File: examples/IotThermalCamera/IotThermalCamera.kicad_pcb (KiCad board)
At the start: 4 copper layers, 48 x 37 mm, 53 parts

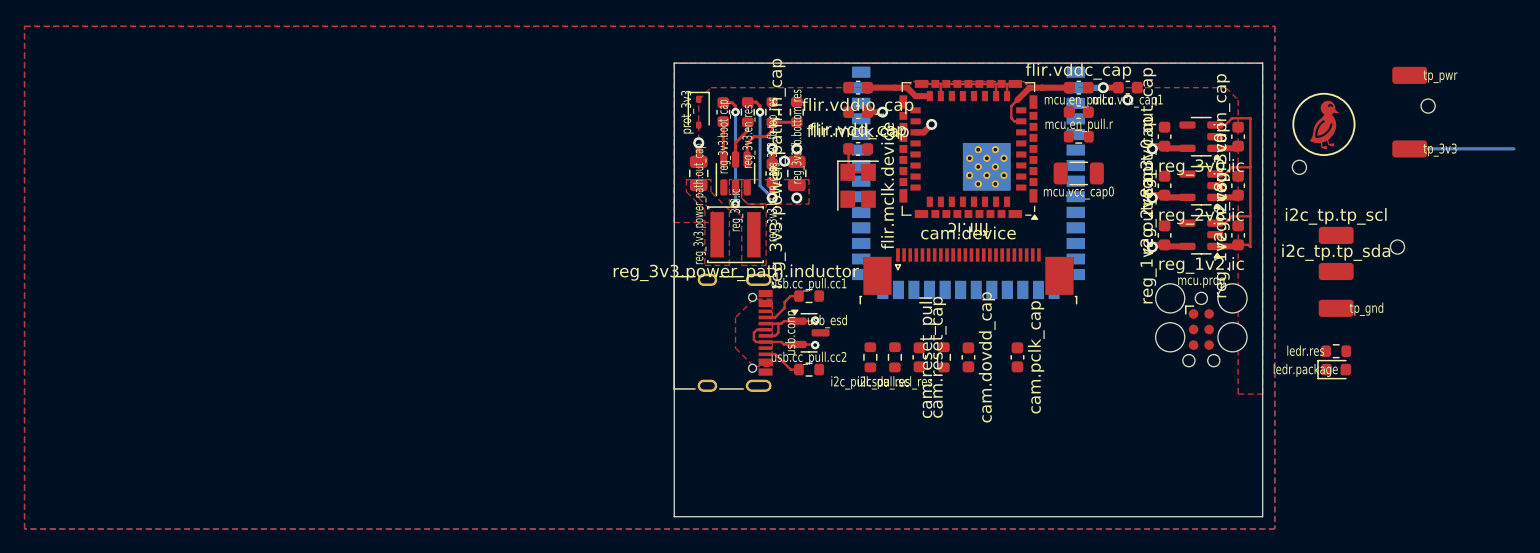
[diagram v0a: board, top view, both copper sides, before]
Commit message: Update IotThermalCamera.kicad_pcb
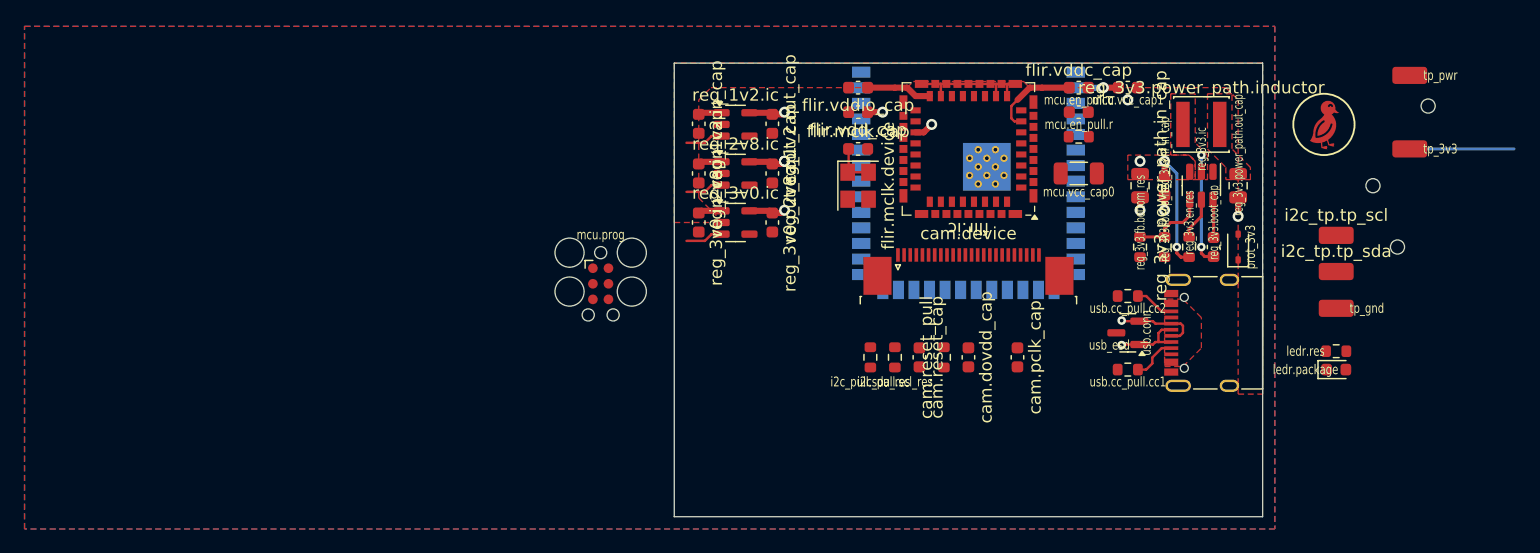
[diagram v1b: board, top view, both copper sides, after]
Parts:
- moved mcu.prog 49.1 mm to (120.0, 111.0)
- moved prot_3v3 45.4 mm to (172.0, 108.0), turned to 90 degrees
- moved reg_1v2.in_cap 44.9 mm to (128.0, 98.0), turned to -90 degrees
- moved reg_3v0.in_cap 44.6 mm to (128.0, 106.0), turned to -90 degrees
- moved reg_2v8.in_cap 44.0 mm to (128.0, 102.0), turned to -90 degrees
- moved reg_3v3.power_path.out_cap 44.0 mm to (172.0, 103.0), turned to -90 degrees
- moved reg_3v3.boot_cap 41.5 mm to (170.0, 108.0), turned to -90 degrees
- moved usb.conn 40.4 mm to (170.2, 115.0), turned to 90 degrees
- moved reg_1v2.ic 39.1 mm to (131.0, 98.0), turned to 0 degrees
- moved reg_3v3.power_path.inductor 39.1 mm to (169.0, 98.0), turned to 0 degrees
- moved reg_3v0.ic 38.6 mm to (131.0, 106.0), turned to 0 degrees
- moved reg_2v8.ic 38.0 mm to (131.0, 102.0), turned to 0 degrees
- moved reg_3v3.ic 38.0 mm to (169.0, 103.0), turned to -90 degrees
- moved reg_3v3.en_res 37.6 mm to (168.0, 108.0), turned to 90 degrees
- moved reg_3v3.fb.top_res 33.8 mm to (166.0, 108.0), turned to 90 degrees
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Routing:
- net Tv3v3: track 30.1 -> 18.5 mm
- net Tv2v8: vias 3 -> 4
- net Tgnd: vias 5 -> 4
